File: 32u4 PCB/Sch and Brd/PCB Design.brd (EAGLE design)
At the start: 95.8 x 64.6 mm, 54 parts, among them J1 AVR_SPI_PROG_3X2PTH, J2 AMP FCI 10103594-0001LF, Q1 16MHz, U1 ATMEGA32U4-AU

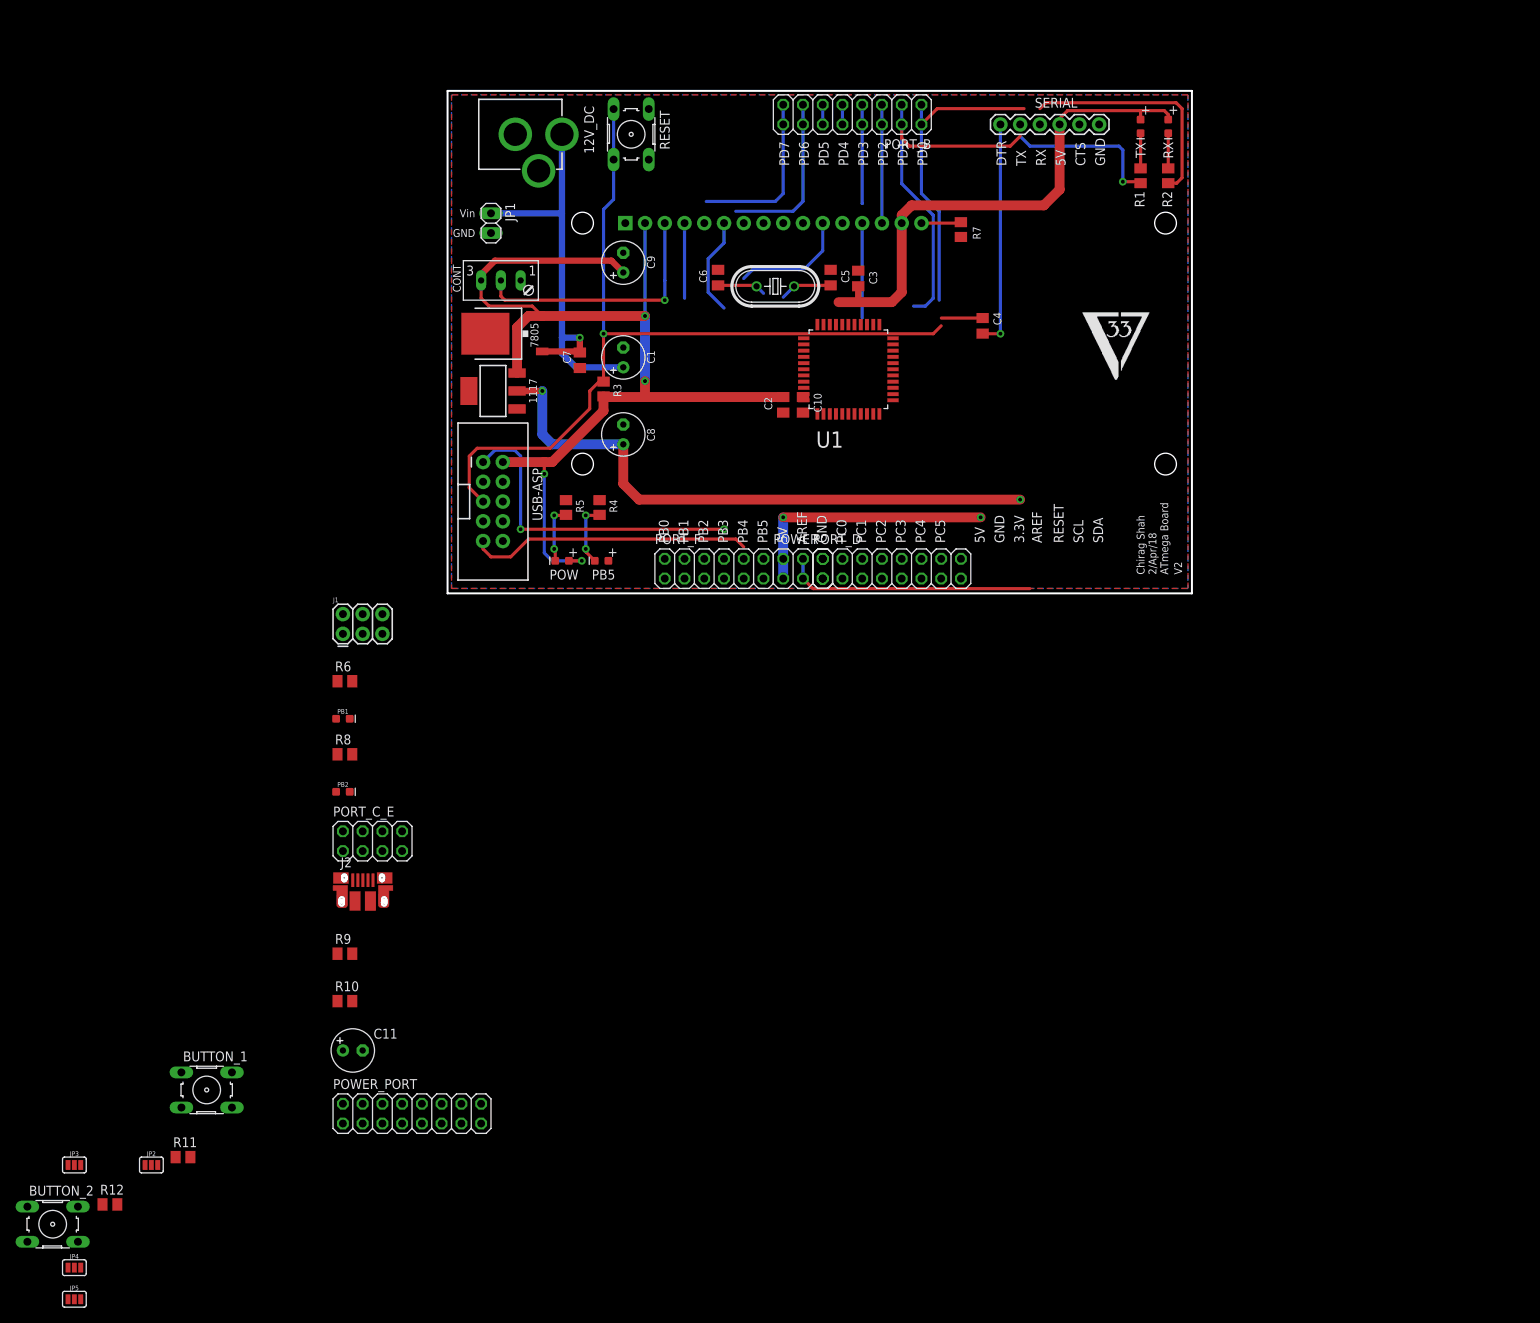
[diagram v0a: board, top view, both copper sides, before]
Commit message: Started routinng
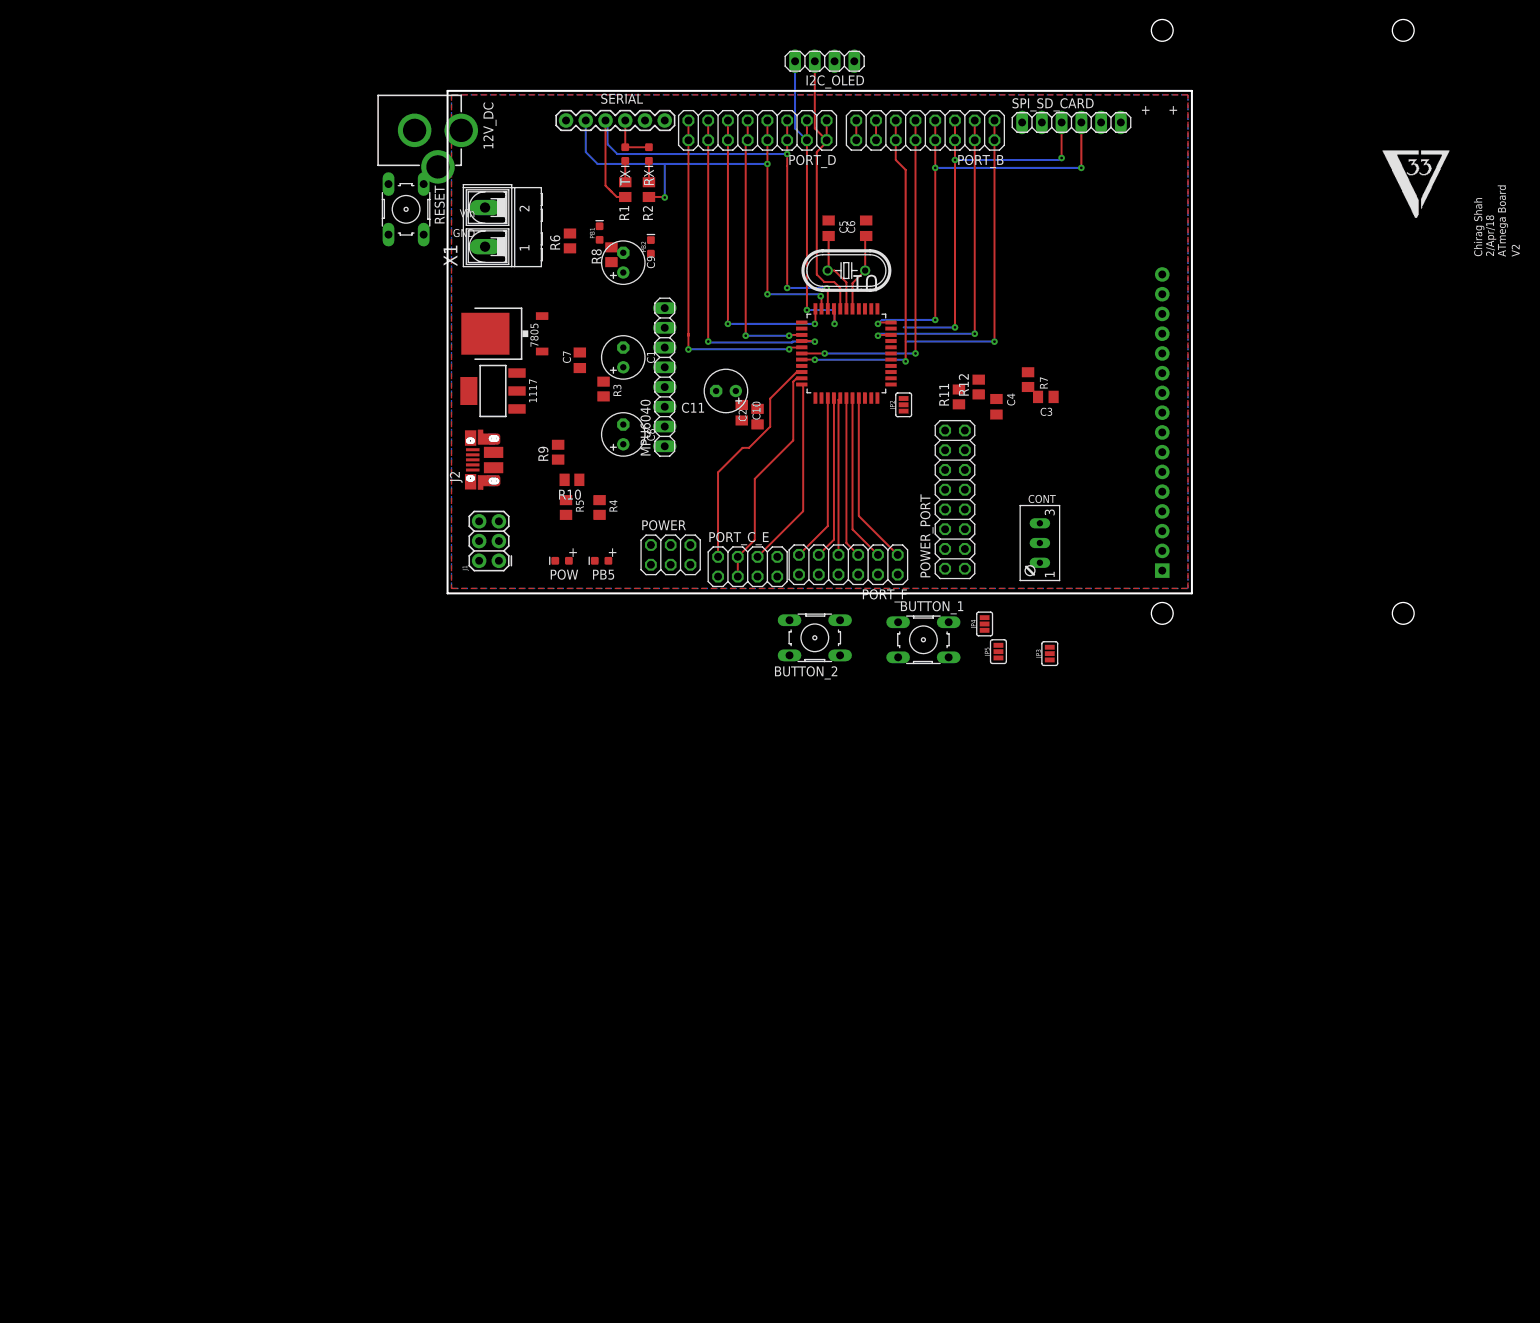
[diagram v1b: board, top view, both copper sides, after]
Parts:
- removed JP1: (no value), pinhead:1X02
- removed USB-ASP: AVR_SPI_PROG_5X2PTH2, SparkFun-Connectors:2X5-SHROUDED
- added I2C_OLED: (no value), pinhead:1X04
- added MPU6040: (no value), pinhead:1X08
- added SPI_SD_CARD: (no value), pinhead:1X06
- added X1: (no value), con-ptr500:AK500/2-H
- moved R12 153.5 mm to (75.7, 32.3), turned to 90 degrees
- moved JP5 145.2 mm to (78.2, -1.78), turned to 90 degrees
- moved JP4 143.4 mm to (76.5, 1.78), turned to 90 degrees
- moved JP3 141.7 mm to (84.8, -2.03), turned to 90 degrees
- moved R11 139.7 mm to (73.2, 31.0), turned to 90 degrees
- moved JP2 137.6 mm to (66.0, 30.0), turned to 90 degrees
- moved BUTTON_2 123.7 mm to (54.6, 0.00), turned to 180 degrees
- moved BUTTON_1 108.9 mm to (68.6, -0.25)
- moved POWER_PORT 105.4 mm to (72.6, 17.8), turned to 90 degrees
- moved C11 97.5 mm to (43.2, 31.8), turned to 180 degrees
- moved PB2 80.5 mm to (33.5, 50.3), turned to 90 degrees
- moved CONT 75.4 mm to (82.3, 12.2), turned to 270 degrees
- moved R10 73.1 mm to (23.4, 20.3), turned to 180 degrees
- moved R8 72.8 mm to (28.4, 49.3), turned to 90 degrees
- moved PB1 70.7 mm to (26.9, 52.1), turned to 90 degrees
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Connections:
- net PD2 renamed PD2/RXD1
- net PD3 renamed PD3/TXD1
- net PF4 renamed PF4/TCK
- net PF5 renamed PF5/TMS
- net PF6 renamed PF6/TDO
- net PF7 renamed PF7/TDI
- removed net PB1: J1.3, PORT_B.3, PORT_B.4, U1.9, USB-ASP.7
- removed net PB2: J1.4, PORT_B.5, PORT_B.6, U1.10, USB-ASP.1
- removed net PB3: J1.1, PORT_B.7, PORT_B.8, U1.11, USB-ASP.9
- removed net PD0: PORT_D.1, PORT_D.2, U1.18
- removed net PD1: PORT_D.3, PORT_D.4, U1.19
- new net AD0: MPU6040.7
- new net CS: SPI_SD_CARD.1
- new net INT: MPU6040.8
- new net PB1/SCK: J1.3, PORT_B.3, PORT_B.4, SPI_SD_CARD.2, U1.9
- new net PB2/MOSI: J1.4, PORT_B.5, PORT_B.6, SPI_SD_CARD.3, U1.10
- new net PB3/MISO: J1.1, PORT_B.7, PORT_B.8, SPI_SD_CARD.4, U1.11
- new net PD0/SCL: I2C_OLED.3, MPU6040.3, PORT_D.1, PORT_D.2, U1.18
- new net PD1/SDA: I2C_OLED.4, MPU6040.4, PORT_D.3, PORT_D.4, U1.19
- new net XCL: MPU6040.6
- new net XDA: MPU6040.5
- net +12V: now also X1.2; no longer JP1.1
- net +5V: now also I2C_OLED.2, MPU6040.1, SPI_SD_CARD.5; no longer USB-ASP.2
- net GND: now also I2C_OLED.1, MPU6040.2, SPI_SD_CARD.6, X1.1; no longer JP1.2, USB-ASP.10, USB-ASP.4, USB-ASP.6, USB-ASP.8
- net RESET: no longer USB-ASP.5
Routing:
- net +5V: track 237.2 -> 6.49 mm, vias 6 -> 0
- net RESET: track 113.9 -> 0.00 mm, vias 1 -> 0
- net 3.3V: track 76.8 -> 0.00 mm, vias 2 -> 0
- net PB3/MISO: track 0.00 -> 59.6 mm, vias 0 -> 4
- net PB2: track 56.6 -> 0.00 mm, vias 2 -> 0
- net +12V: track 55.1 -> 0.00 mm, vias 1 -> 0
- net PB2/MOSI: track 0.00 -> 51.6 mm, vias 0 -> 3
- net PB3: track 49.0 -> 0.00 mm
- net PD2/RXD1: track 20.4 -> 68.0 mm, vias 1 -> 3
- net PB1: track 47.5 -> 0.00 mm
- net PD7: track 0.00 -> 44.4 mm, vias 0 -> 2
- net PD6: track 0.00 -> 44.0 mm, vias 0 -> 2
- net PB5: track 2.55 -> 45.0 mm, vias 0 -> 2
- net PD1/SDA: track 0.00 -> 42.3 mm, vias 0 -> 2
- net PB4: track 2.55 -> 44.6 mm, vias 0 -> 2
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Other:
- board text removed: "3.3V"
- board text removed: "5V"
- board text removed: "AREF"
- board text removed: "CTS"
- board text removed: "DTR"
- board text removed: "PB0"
- board text removed: "PB1"
- board text removed: "PB2"
- board text removed: "PB3"
- board text removed: "PB4"
- board text removed: "PB5"
- board text removed: "PC0"
- board text removed: "PC1"
- board text removed: "PC2"
- board text removed: "PC3"
- board text removed: "PC4"
- board text removed: "PC5"
- board text removed: "PD0"
- board text removed: "PD1"
- board text removed: "PD2"
- board text removed: "PD3"
- board text removed: "PD4"
- board text removed: "PD5"
- board text removed: "PD6"
- board text removed: "PD7"
- board text removed: "RESET"
- board text removed: "RX"
- board text removed: "SCL"
- board text removed: "SDA"
- board text removed: "TX"

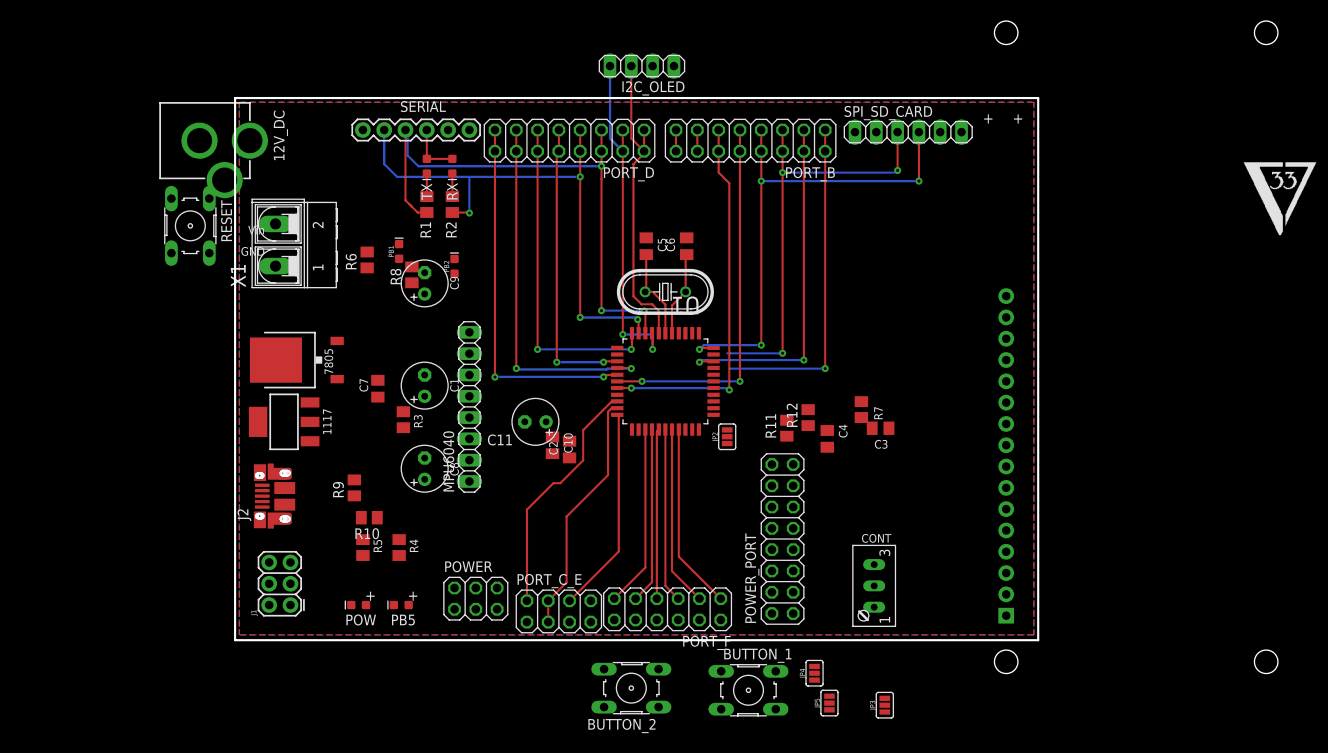
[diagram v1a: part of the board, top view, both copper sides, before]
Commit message: Started routinng
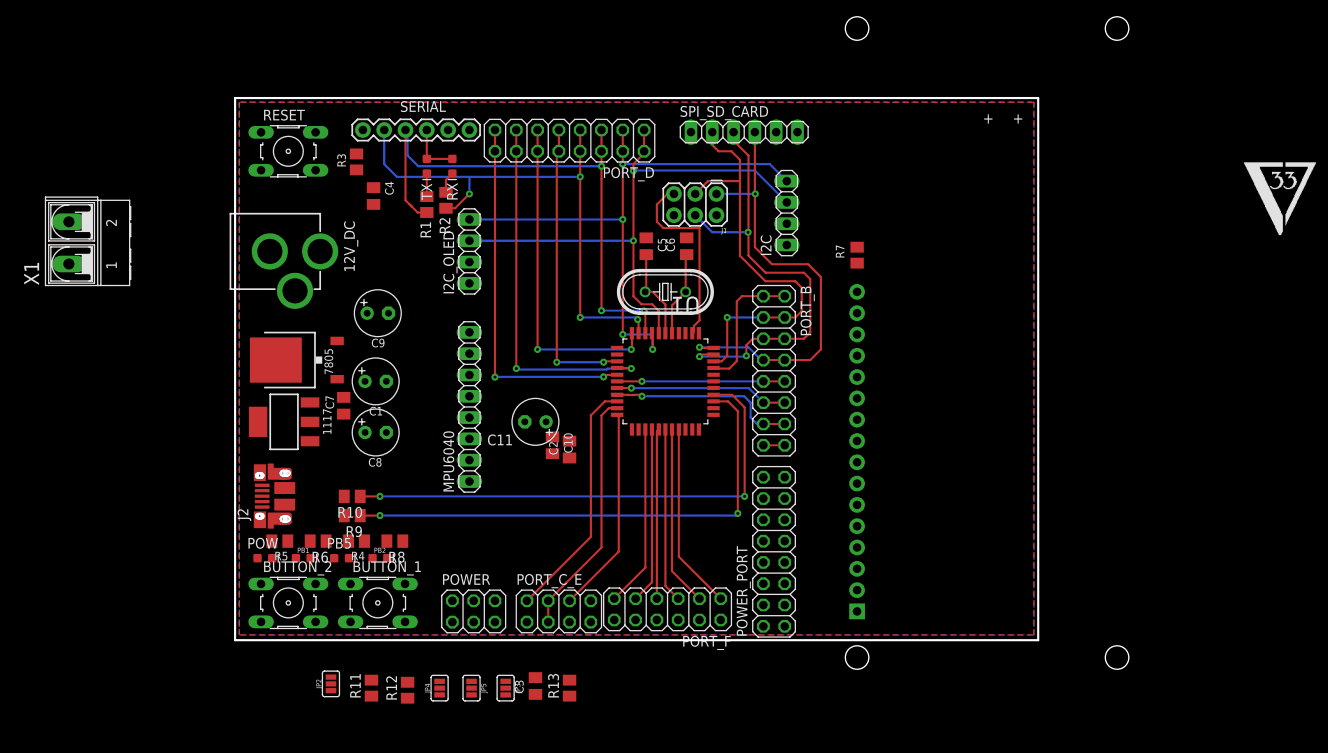
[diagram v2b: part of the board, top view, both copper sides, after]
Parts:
- removed CONT: 50k, pot:S64W
- added I2C: (no value), pinhead:1X04
- added R13: 220, resistor:M0805
- moved J1 70.6 mm to (64.8, 58.9), turned to 180 degrees
- moved C4 61.4 mm to (23.9, 58.7)
- moved R11 58.4 mm to (23.6, 0.00)
- moved R12 57.8 mm to (27.9, -0.25)
- moved JP2 55.7 mm to (18.8, 0.51)
- moved C3 51.4 mm to (43.2, 0.25), turned to 270 degrees
- moved BUTTON_1 45.4 mm to (24.4, 10.2)
- moved JP3 45.3 mm to (39.6, 0.00), turned to 270 degrees
- moved JP4 44.7 mm to (31.8, 0.00)
- moved JP5 42.7 mm to (35.6, 0.00), turned to 270 degrees
- moved BUTTON_2 42.1 mm to (13.7, 10.2), turned to 0 degrees
- moved PB1 38.3 mm to (15.5, 15.5), turned to 0 degrees
- moved PB2 35.9 mm to (24.6, 15.5), turned to 0 degrees
- moved R6 34.0 mm to (17.3, 17.5), turned to 180 degrees
- moved R8 31.8 mm to (26.4, 17.5), turned to 180 degrees
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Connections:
- net +12V: no longer X1.2
- net +5V: now also I2C.2; no longer CONT.E
- net GND: now also I2C.1, R13.1; no longer CONT.A, X1.1
- net N$6: now also R13.2; no longer CONT.S
- net PD0/SCL: now also I2C.3
- net PD1/SDA: now also I2C.4
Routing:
- net N$15: track 0.00 -> 60.8 mm, vias 0 -> 2
- net N$13: track 0.00 -> 60.7 mm, vias 0 -> 2
- net PD0/SCL: track 37.5 -> 66.2 mm, vias 0 -> 2
- net PD1/SDA: track 42.3 -> 70.2 mm, vias 2 -> 4
- net PB4: track 44.6 -> 20.0 mm, vias 2 -> 1
- net PB5: track 45.0 -> 20.7 mm, vias 2 -> 1
- net PB0: track 40.0 -> 17.0 mm, vias 1 -> 0
- net RESET: track 0.00 -> 22.9 mm
- net PB6: track 2.54 -> 22.5 mm, vias 0 -> 1
- net PB1/SCK: track 41.7 -> 51.2 mm, vias 2 -> 1
- net PB3/MISO: track 59.6 -> 53.7 mm, vias 4 -> 2
- net PB2/MOSI: track 51.6 -> 54.6 mm
- net PC7: track 29.3 -> 30.2 mm
- net PD3/TXD1: track 65.4 -> 64.6 mm
- net PC6: track 29.1 -> 29.7 mm
- added copper zone on layer 16, net +5V
- removed copper zone on layer 16, net GND
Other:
- board text removed: "GND"
- board text removed: "Vin"
